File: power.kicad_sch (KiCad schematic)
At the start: 15 parts, among them U8 PLM62440APPQRJRTQ1

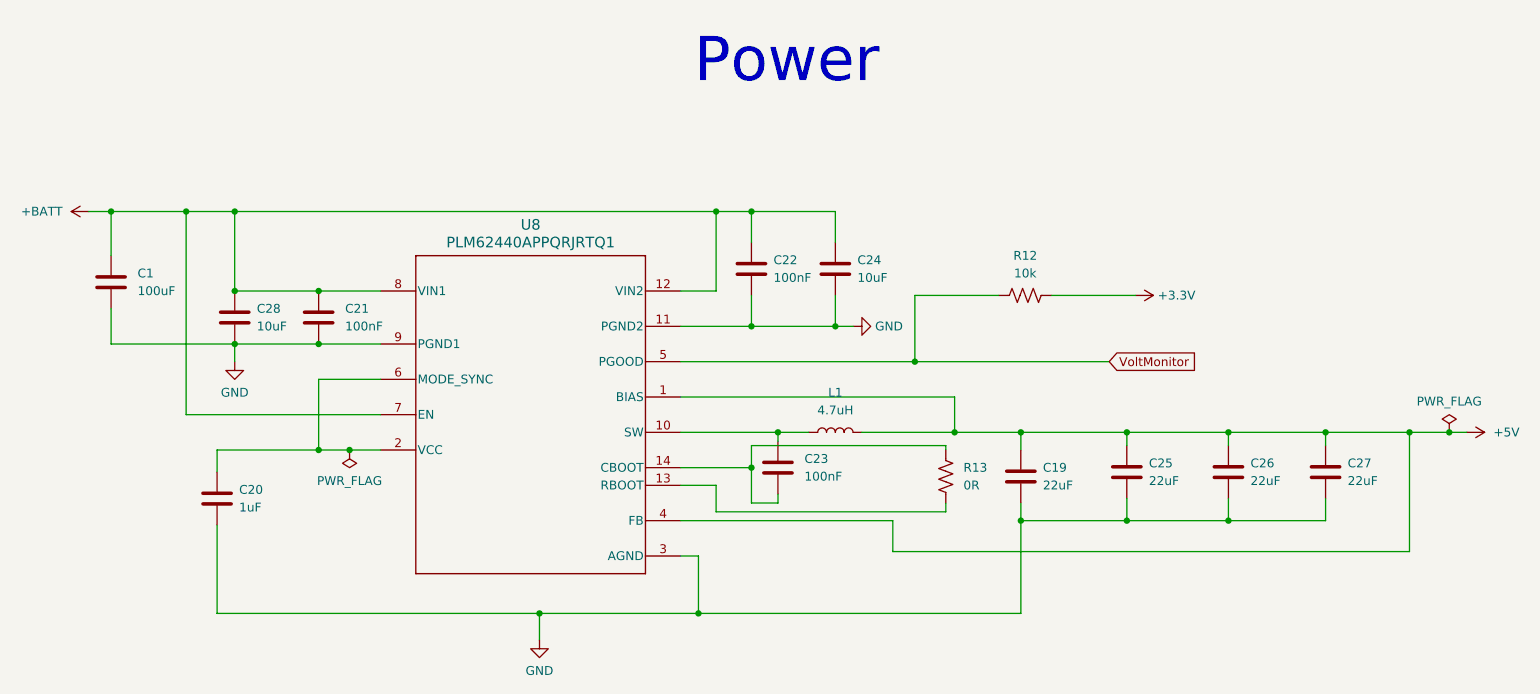
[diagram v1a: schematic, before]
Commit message: simple-fixes
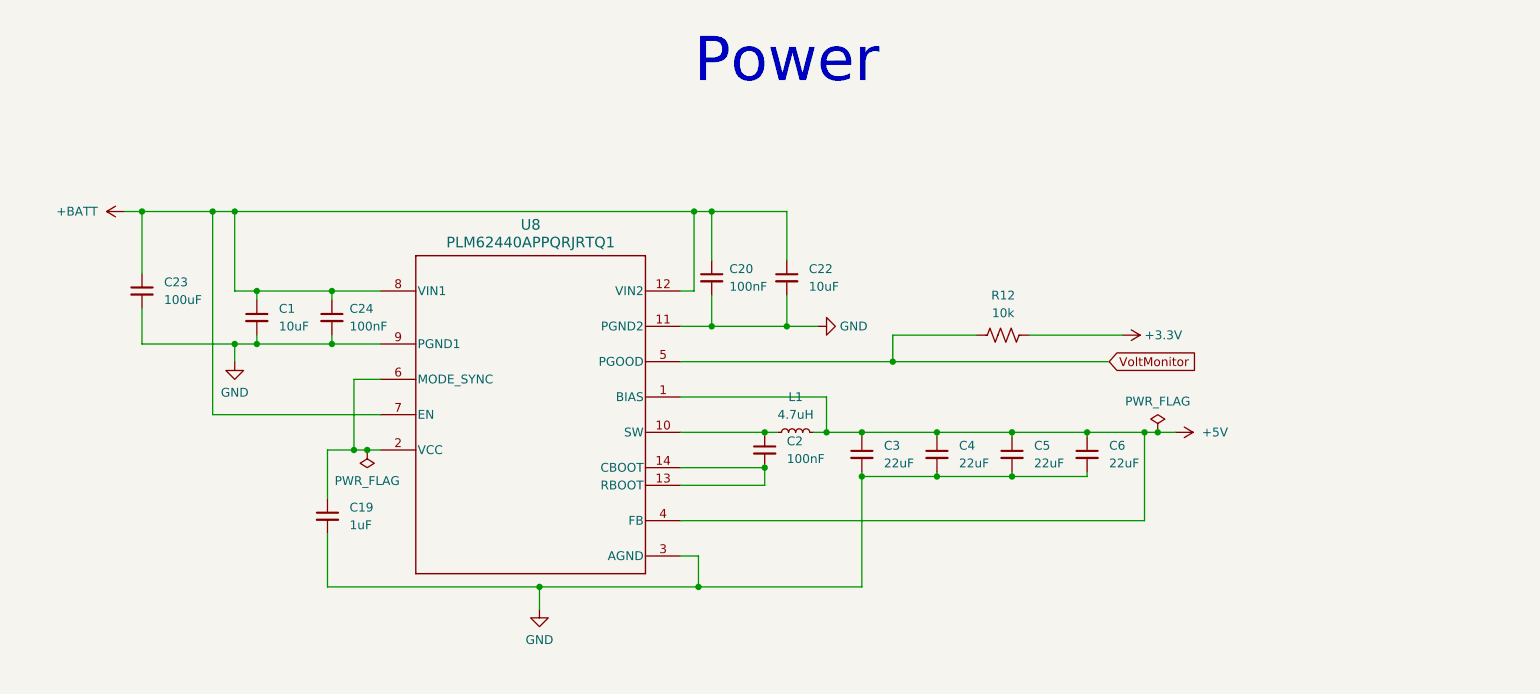
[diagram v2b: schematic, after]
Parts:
- removed C1: 100uF, Capacitor_SMD:C_0201_0603Metric, symbol Device:C
- removed C19, C25, C26, C27: 22uF, Capacitor_SMD:C_0603_1608Metric, symbol Device:C
- removed C20: 1uF, symbol Device:C
- removed C21, C22, C23: 100nF, symbol Device:C
- removed C24, C28: 10uF, symbol Device:C
- removed L1: 4.7uH, symbol Device:L
- removed R13: 0R, symbol Device:R_US
- added C1, C22: 10uF, Capacitor_SMD:C_0603_1608Metric, symbol Device:C_Small
- added C19: 1uF, Capacitor_SMD:C_0603_1608Metric, symbol Device:C_Small
- added C2, C20, C24: 100nF, Capacitor_SMD:C_0603_1608Metric, symbol Device:C_Small
- added C23: 100uF, Capacitor_SMD:C_0603_1608Metric, symbol Device:C_Small
- added C3, C4, C5, C6: 22uF, Capacitor_SMD:C_0603_1608Metric, symbol Device:C_Small
- added L1: 4.7uH, Inductor_SMD:L_0603_1608Metric, symbol Device:L_Small
- R12: footprint (none) -> Resistor_SMD:R_0603_1608Metric
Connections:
- net +5V: now also C3.1, C4.1, C5.1, C6.1, L1.2
- net +BATT: now also C1.1, C20.1, C22.1, C23.1, C24.1
- net GND: now also C1.2, C19.2, C20.2, C22.2, C23.2, C24.2, C3.2, C4.2, C5.2, C6.2
- net at U8.14 (CBOOT): now also U8.13 (RBOOT), C2.2
- net at U8.10 (SW): now also C2.1, L1.1
- net at U8.2 (VCC), U8.6 (MODE_SYNC): now also C19.1
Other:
- moved on the sheet: R12
